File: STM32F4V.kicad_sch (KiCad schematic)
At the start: 18 parts, among them SW1 STMRESET, U1 STM32F407VGTx, Y1 25MHz

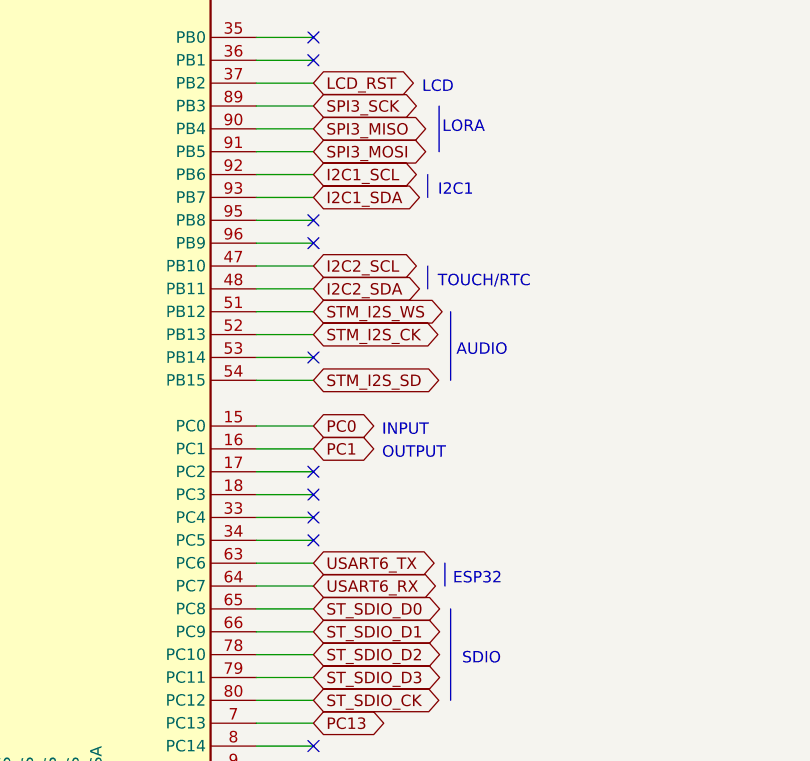
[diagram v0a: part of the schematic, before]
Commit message: Add files via upload
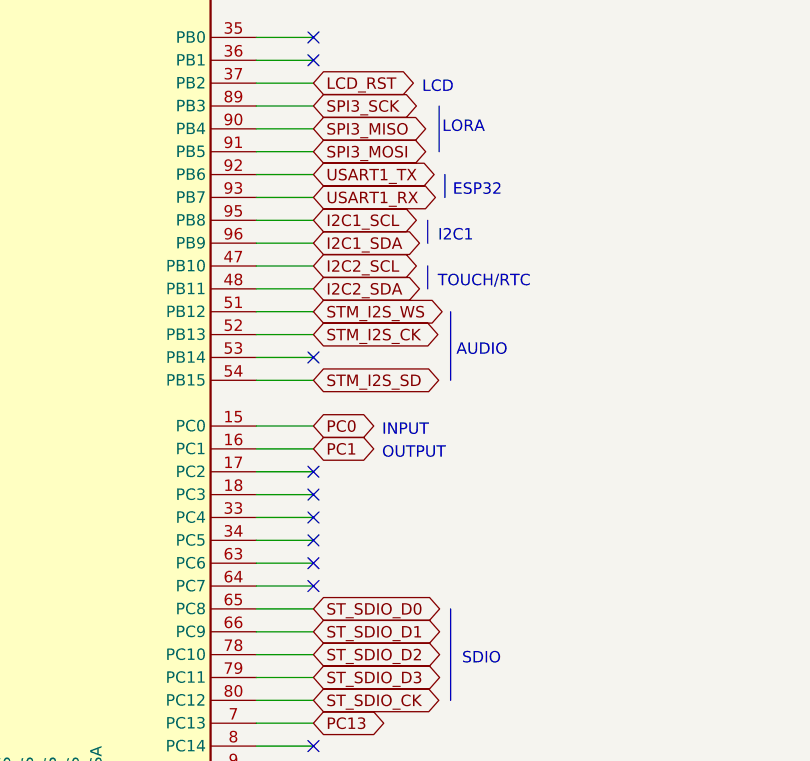
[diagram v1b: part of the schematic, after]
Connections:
- net I2C1_SCL: now also U1.95 (PB8); no longer U1.92 (PB6)
- net I2C1_SDA: now also U1.96 (PB9); no longer U1.93 (PB7)
- net USART6_RX: no longer names the net of U1.64 (PC7)
- net USART6_TX: no longer names the net of U1.63 (PC6)
- new net USART1_RX: U1.93 (PB7)
- new net USART1_TX: U1.92 (PB6)
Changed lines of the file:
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@@
   )
   (no_connect (at 107.95 120.65))
+  (no_connect (at 107.95 181.61))
   (no_connect (at 107.95 176.53))
   (no_connect (at 107.95 171.45))
@@
   (no_connect (at 107.95 156.21))
   (no_connect (at 107.95 168.91))
+  (no_connect (at 107.95 179.07))
   (no_connect (at 107.95 173.99))
-  (no_connect (at 107.95 140.97))
-  (no_connect (at 107.95 143.51))
   (no_connect (at 107.95 115.57))
   (no_connect (at 107.95 123.19))
@@
     (stroke (width 0) (type default) (color 0 0 0 0))
   )
-  (bus (pts (xy 122.555 179.07) (xy 122.555 181.61))
+  (bus (pts (xy 122.555 135.89) (xy 122.555 138.43))
     (stroke (width 0) (type default) (color 0 0 0 0))
   )
@@
     (stroke (width 0) (type default) (color 0 0 0 0))
   )
-  (bus (pts (xy 120.65 135.89) (xy 120.65 138.43))
+  (bus (pts (xy 120.65 140.97) (xy 120.65 143.51))
     (stroke (width 0) (type default) (color 0 0 0 0))
   )
@@
     (effects (font (size 1.27 1.27)) (justify right bottom))
   )
-  (text "ESP32" (at 128.905 181.61 180)
+  (text "ESP32" (at 128.905 138.43 180)
     (effects (font (size 1.27 1.27)) (justify right bottom))
   )
@@
     (effects (font (size 1.27 1.27)) (justify left bottom))
   )
-  (text "I2C1" (at 125.73 138.43 180)
+  (text "I2C1" (at 125.73 143.51 180)
     (effects (font (size 1.27 1.27)) (justify right bottom))
   )
@@
     )
   )
-  (global_label "I2C1_SCL" (shape bidirectional) (at 107.95 135.89 0) (fields_autoplaced)
-    (effects (font (size 1.27 1.27)) (justify left))
-    (property "Intersheet References" "${INTERSHEET_REFS}" (id 0) (at 119.1321 135.8106 0)
+  (global_label "I2C1_SCL" (shape bidirectional) (at 107.95 140.97 0) (fields_autoplaced)
+    (effects (font (size 1.27 1.27)) (justify left))
+    (property "Intersheet References" "${INTERSHEET_REFS}" (id 0) (at 119.1321 140.8906 0)
       (effects (font (size 1.27 1.27)) (justify left) hide)
     )
@@
     )
   )
-  (global_label "I2C1_SDA" (shape bidirectional) (at 107.95 138.43 0) (fields_autoplaced)
-    (effects (font (size 1.27 1.27)) (justify left))
-    (property "Intersheet References" "${INTERSHEET_REFS}" (id 0) (at 119.1926 138.3506 0)
+  (global_label "I2C1_SDA" (shape bidirectional) (at 107.95 143.51 0) (fields_autoplaced)
+    (effects (font (size 1.27 1.27)) (justify left))
+    (property "Intersheet References" "${INTERSHEET_REFS}" (id 0) (at 119.1926 143.4306 0)
       (effects (font (size 1.27 1.27)) (justify left) hide)
     )
@@
     )
   )
-  (global_label "USART6_RX" (shape bidirectional) (at 107.95 181.61 0) (fields_autoplaced)
-    (effects (font (size 1.27 1.27)) (justify left))
-    (property "Intersheet References" "${INTERSHEET_REFS}" (id 0) (at 120.886 181.5306 0)
+  (global_label "USART1_RX" (shape bidirectional) (at 107.95 138.43 0) (fields_autoplaced)
+    (effects (font (size 1.27 1.27)) (justify left))
+    (property "Intersheet References" "${INTERSHEET_REFS}" (id 0) (at 120.886 138.3506 0)
       (effects (font (size 1.27 1.27)) (justify left) hide)
     )
@@
     )
   )
-  (global_label "USART6_TX" (shape bidirectional) (at 107.95 179.07 0) (fields_autoplaced)
-    (effects (font (size 1.27 1.27)) (justify left))
-    (property "Intersheet References" "${INTERSHEET_REFS}" (id 0) (at 120.5836 178.9906 0)
-      (effects (font (size 1.27 1.27)) (justify left) hide)
-    )
+  (global_label "USART1_TX" (shape bidirectional) (at 107.95 135.89 0) (fields_autoplaced)
+    (effects (font (size 1.27 1.27)) (justify left))
+    (property "Intersheet References" "${INTERSHEET_REFS}" (id 0) (at 120.5836 135.8106 0)
+      (effects (font (size 1.27 1.27)) (justify left) hide)
+    )

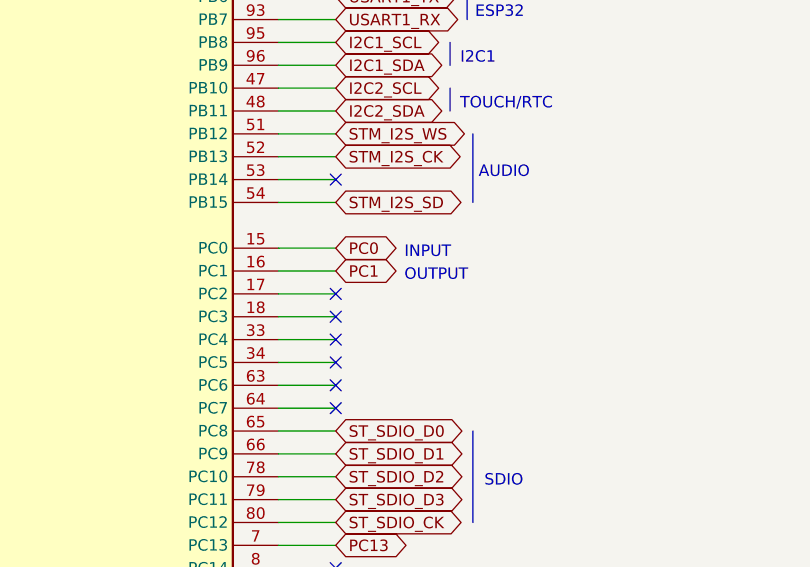
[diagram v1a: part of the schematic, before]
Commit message: Add files via upload
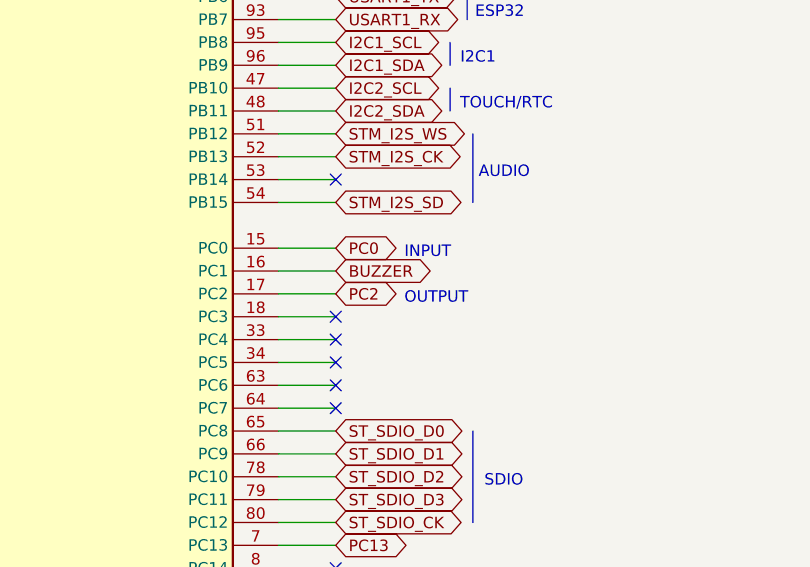
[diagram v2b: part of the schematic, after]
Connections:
- net PC2: now reaches U1.17 (PC2)
- net PC1 renamed BUZZER
- no-connect marks 15 -> 14
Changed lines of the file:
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@@
   (no_connect (at 107.95 171.45))
   (no_connect (at 71.12 69.85))
+  (no_connect (at 107.95 115.57))
   (no_connect (at 107.95 199.39))
   (no_connect (at 107.95 201.93))
@@
   (no_connect (at 49.53 191.77))
   (no_connect (at 107.95 156.21))
-  (no_connect (at 107.95 168.91))
   (no_connect (at 107.95 179.07))
   (no_connect (at 107.95 173.99))
-  (no_connect (at 107.95 115.57))
   (no_connect (at 107.95 123.19))
   (wire (pts (xy 101.6 113.03) (xy 107.95 113.03))
@@
     (effects (font (size 1.27 1.27)) (justify right bottom))
   )
-  (text "OUTPUT" (at 115.57 167.64 0)
+  (text "OUTPUT" (at 115.57 170.18 0)
     (effects (font (size 1.27 1.27)) (justify left bottom))
   )
@@
     )
   )
-  (global_label "PC1" (shape bidirectional) (at 107.95 166.37 0) (fields_autoplaced)
-    (effects (font (size 1.27 1.27)) (justify left))
-    (property "Intersheet References" "${INTERSHEET_REFS}" (id 0) (at 114.1126 166.2906 0)
+  (global_label "PC2" (shape bidirectional) (at 107.95 168.91 0) (fields_autoplaced)
+    (effects (font (size 1.27 1.27)) (justify left))
+    (property "Intersheet References" "${INTERSHEET_REFS}" (id 0) (at 114.1126 168.8306 0)
       (effects (font (size 1.27 1.27)) (justify left) hide)
     )
@@
     )
   )
+  (global_label "BUZZER" (shape bidirectional) (at 107.95 166.37 0) (fields_autoplaced)
+    (effects (font (size 1.27 1.27)) (justify left))
+    (property "Intersheet References" "${INTERSHEET_REFS}" (id 0) (at 117.8017 166.2906 0)
+      (effects (font (size 1.27 1.27)) (justify left) hide)
+    )
+  )
